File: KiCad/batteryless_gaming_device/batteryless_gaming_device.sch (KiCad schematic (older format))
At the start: 0 parts

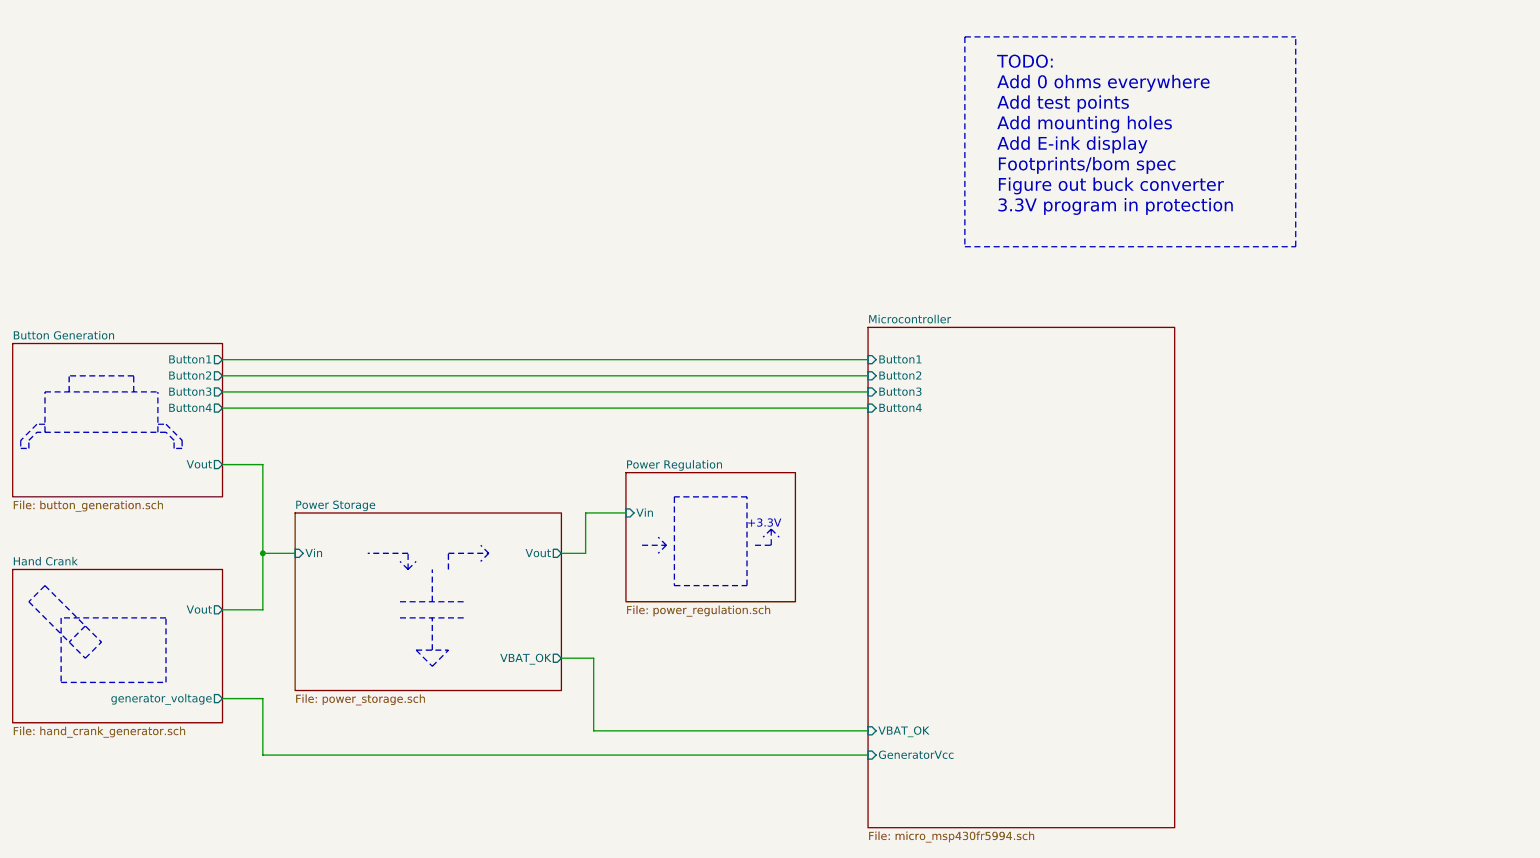
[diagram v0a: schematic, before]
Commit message: k
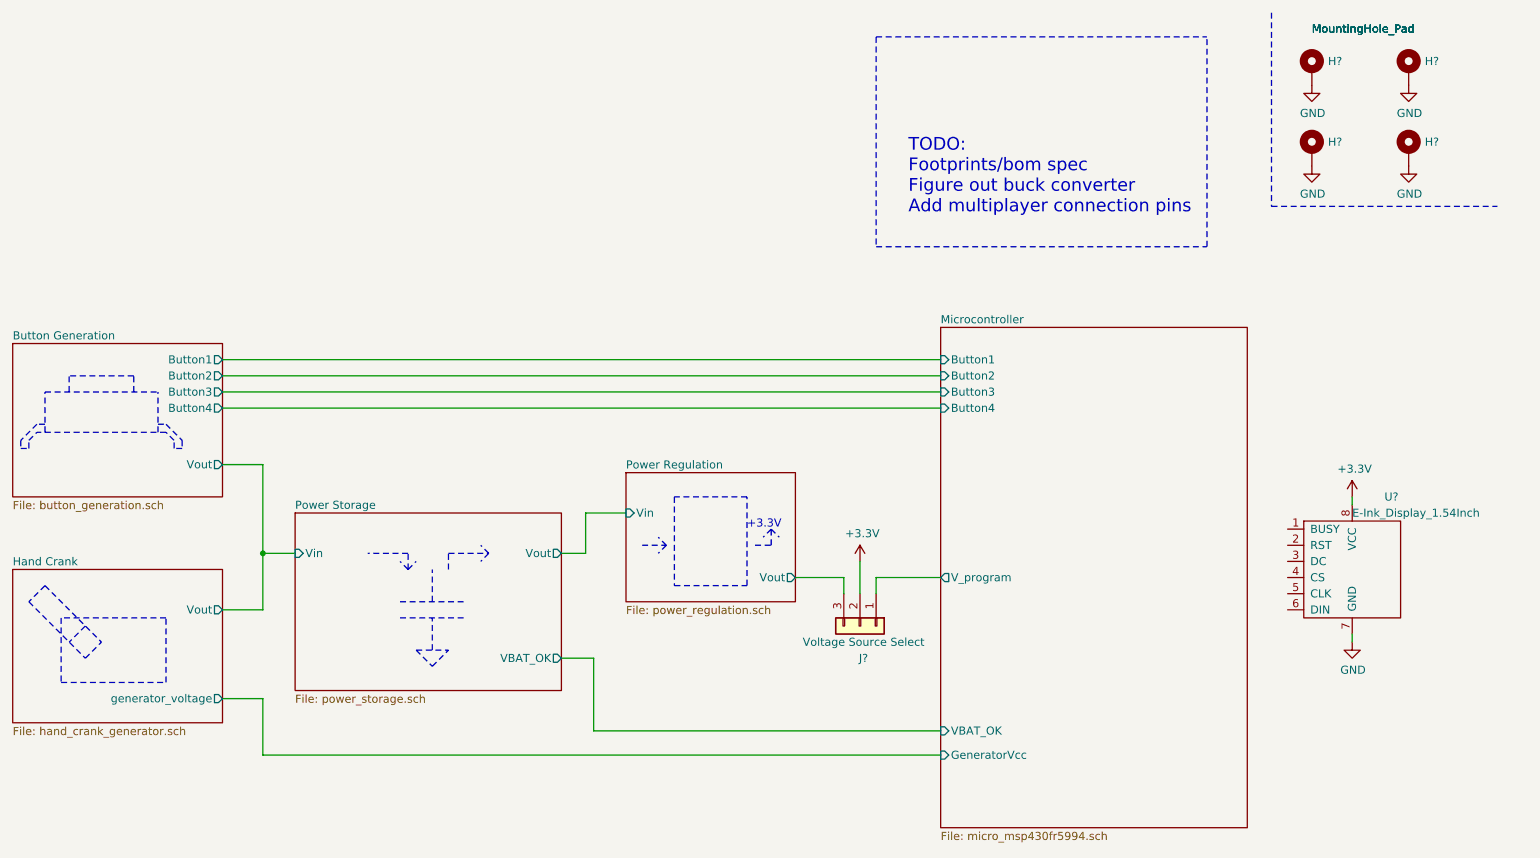
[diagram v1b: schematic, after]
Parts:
- added H? (x4): MountingHole_Pad, symbol Mechanical:MountingHole_Pad
- added J?: Voltage Source Select, symbol Connector_Generic:Conn_01x03
- added U?: E-Ink_Display_1.54Inch, symbol batteryless_gaming_device-rescue:E-Ink_Display_1.54Inch
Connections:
- new net +3V3: J?.2 (Pin_2), U?.8 (VCC)
- new net GND: H?.1, H?.1, H?.1, H?.1, U?.7 (GND)
- new net Microcontroller/V_program: J?.1 (Pin_1)
- new net Power Regulation/Vout: J?.3 (Pin_3)
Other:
- note added: "TODO:\nFootprints/bom spec\nFigure out buck converter\nAdd multiplayer connection pins"
- note removed: "TODO:\nAdd 0 ohms everywhere\nAdd test points\nAdd mounting holes\nAdd E-ink display\nFootprints/bom spec\nFigure out buck converter\n3.3V program in protection"
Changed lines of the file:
@@
 $EndSheet
 $Sheet
-S 6600 2450 1900 3100
+S 7050 2450 1900 3100
 U 61926AE2
 F0 "Microcontroller" 50
 F1 "micro_msp430fr5994.sch" 50
-F2 "Button1" I L 6600 2650 50
-F3 "Button2" I L 6600 2750 50
-F4 "Button3" I L 6600 2850 50
-F5 "Button4" I L 6600 2950 50
-F6 "GeneratorVcc" I L 6600 5100 50
-F7 "VBAT_OK" I L 6600 4950 50
+F2 "Button1" I L 7050 2650 50
+F3 "Button2" I L 7050 2750 50
+F4 "Button3" I L 7050 2850 50
+F5 "Button4" I L 7050 2950 50
+F6 "GeneratorVcc" I L 7050 5100 50
+F7 "VBAT_OK" I L 7050 4950 50
+F8 "V_program" O L 7050 4000 50
 $EndSheet
 Wire Wire Line
@@
 F1 "power_regulation.sch" 50
 F2 "Vin" I L 5100 3600 50
+F3 "Vout" O R 6150 4000 50
 $EndSheet
 Wire Wire Line
@@
 	5200 3800 5350 3800
 Wire Wire Line
-	2600 2950 6600 2950
-Wire Wire Line
-	2600 2850 6600 2850
-Wire Wire Line
-	2600 2750 6600 2750
-Wire Wire Line
-	2600 2650 6600 2650
+	2600 2950 7050 2950
+Wire Wire Line
+	2600 2850 7050 2850
+Wire Wire Line
+	2600 2750 7050 2750
+Wire Wire Line
+	2600 2650 7050 2650
 Wire Wire Line
 	2600 4750 2850 4750
@@
 	2850 4750 2850 5100
 Wire Wire Line
-	2850 5100 6600 5100
+	2850 5100 7050 5100
 Wire Wire Line
 	4700 4500 4900 4500
@@
 	4900 4500 4900 4950
 Wire Wire Line
-	4900 4950 6600 4950
-Text Notes 7400 1750 0    79   ~ 0
-TODO:\nAdd 0 ohms everywhere\nAdd test points\nAdd mounting holes\nAdd E-ink display\nFootprints/bom spec\nFigure out buck converter\n3.3V program in protection
-Wire Notes Line
-	7200 650  7200 1950
-Wire Notes Line
-	7200 1950 9250 1950
-Wire Notes Line
-	9250 1950 9250 650
-Wire Notes Line
-	7200 650  9250 650
+	4900 4950 7050 4950
+Text Notes 6850 1750 0    79   ~ 0
+TODO:\nFootprints/bom spec\nFigure out buck converter\nAdd multiplayer connection pins
+Wire Notes Line
+	6650 650  6650 1950
+Wire Notes Line
+	6650 1950 8700 1950
+Wire Notes Line
+	8700 1950 8700 650
+Wire Notes Line
+	6650 650  8700 650
+$Comp
+L Connector_Generic:Conn_01x03 J?
+U 1 1 61979531
+P 6550 4300
+F 0 "J?" V 6750 4350 50  0000 R CNN
+F 1 "Voltage Source Select" V 6650 4700 50  0000 R CNN
+F 2 "" H 6550 4300 50  0001 C CNN
+F 3 "~" H 6550 4300 50  0001 C CNN
+	1    6550 4300
+	0    1    1    0
+$EndComp
+Wire Wire Line
+	6150 4000 6450 4000
+Wire Wire Line
+	6450 4000 6450 4100
+Wire Wire Line
+	7050 4000 6650 4000
+Wire Wire Line
+	6650 4000 6650 4100
+Wire Wire Line
+	6550 4100 6550 3900
+$Comp
+L power:+3.3V #PWR?
+U 1 1 61980457
+P 6550 3900
+AR Path="/61926AE2/61980457" Ref="#PWR?"  Part="1"
+AR Path="/61980457" Ref="#PWR?"  Part="1"
+F 0 "#PWR?" H 6550 3750 50  0001 C CNN
+F 1 "+3.3V" H 6565 4073 50  0000 C CNN
+F 2 "" H 6550 3900 50  0001 C CNN
+F 3 "" H 6550 3900 50  0001 C CNN
+	1    6550 3900
+	1    0    0    -1
+$EndComp
+$Comp
+L batteryless_gaming_device-rescue:E-Ink_Display_1.54Inch U?
+U 1 1 61986176
+P 9550 3650
+F 0 "U?" H 9800 3800 50  0000 L CNN
+F 1 "E-Ink_Display_1.54Inch" H 9600 3700 50  0000 L CNN
+F 2 "" H 9550 4150 50  0001 C CNN
+F 3 "" H 9550 4150 50  0001 C CNN
+	1    9550 3650
+	1    0    0    -1
+$EndComp
+$Comp
+L power:GND #PWR?
+U 1 1 61988A0E
+P 9600 4400
+AR Path="/61926AE2/61988A0E" Ref="#PWR?"  Part="1"
+AR Path="/61988A0E" Ref="#PWR?"  Part="1"
+F 0 "#PWR?" H 9600 4150 50  0001 C CNN
+F 1 "GND" H 9605 4227 50  0000 C CNN
+F 2 "" H 9600 4400 50  0001 C CNN
+F 3 "" H 9600 4400 50  0001 C CNN
+	1    9600 4400
+	1    0    0    -1
+$EndComp
+Wire Wire Line
+	9600 4400 9600 4350
+$Comp
+L power:+3.3V #PWR?
+U 1 1 6198A1ED
+P 9600 3500
+AR Path="/61926AE2/6198A1ED" Ref="#PWR?"  Part="1"
+AR Path="/6198A1ED" Ref="#PWR?"  Part="1"
+F 0 "#PWR?" H 9600 3350 50  0001 C CNN
+F 1 "+3.3V" H 9615 3673 50  0000 C CNN
+F 2 "" H 9600 3500 50  0001 C CNN
+F 3 "" H 9600 3500 50  0001 C CNN
+	1    9600 3500
+	1    0    0    -1
+$EndComp
+Wire Wire Line
+	9600 3500 9600 3550
+$Comp
+L Mechanical:MountingHole_Pad H?
+U 1 1 6198BDFD
+P 9350 850
+F 0 "H?" H 9450 899 50  0000 L CNN
+F 1 "MountingHole_Pad" H 9350 1100 50  0000 L CNN
+F 2 "" H 9350 850 50  0001 C CNN
+F 3 "~" H 9350 850 50  0001 C CNN
+	1    9350 850
+	1    0    0    -1
+$EndComp
+$Comp
+L Mechanical:MountingHole_Pad H?
+U 1 1 6198CE4F
+P 9950 850
+F 0 "H?" H 10050 899 50  0000 L CNN
+F 1 "MountingHole_Pad" H 9350 1100 50  0000 L CNN
+F 2 "" H 9950 850 50  0001 C CNN
+F 3 "~" H 9950 850 50  0001 C CNN
+	1    9950 850
+	1    0    0    -1
+$EndComp
+$Comp
+L Mechanical:MountingHole_Pad H?
+U 1 1 6198D15F
+P 9350 1350
+F 0 "H?" H 9450 1399 50  0000 L CNN
+F 1 "MountingHole_Pad" H 9350 2100 50  0000 L CNN
+F 2 "" H 9350 1350 50  0001 C CNN
+F 3 "~" H 9350 1350 50  0001 C CNN
+	1    9350 1350
+	1    0    0    -1
+$EndComp
+$Comp
+L Mechanical:MountingHole_Pad H?
+U 1 1 6198D37A
+P 9950 1350
+F 0 "H?" H 10050 1399 50  0000 L CNN
+F 1 "MountingHole_Pad" H 9350 2100 50  0000 L CNN
+F 2 "" H 9950 1350 50  0001 C CNN
+F 3 "~" H 9950 1350 50  0001 C CNN
+	1    9950 1350
+	1    0    0    -1
+$EndComp
+$Comp
+L power:GND #PWR?
+U 1 1 6198DDE0
+P 9350 1450
+AR Path="/61926AE2/6198DDE0" Ref="#PWR?"  Part="1"
+AR Path="/6198DDE0" Ref="#PWR?"  Part="1"
+F 0 "#PWR?" H 9350 1200 50  0001 C CNN
+F 1 "GND" H 9355 1277 50  0000 C CNN
+F 2 "" H 9350 1450 50  0001 C CNN
+F 3 "" H 9350 1450 50  0001 C CNN
+	1    9350 1450
+	1    0    0    -1
+$EndComp
+$Comp
+L power:GND #PWR?
+U 1 1 6198E313
+P 9950 1450
+AR Path="/61926AE2/6198E313" Ref="#PWR?"  Part="1"
+AR Path="/6198E313" Ref="#PWR?"  Part="1"
+F 0 "#PWR?" H 9950 1200 50  0001 C CNN
+F 1 "GND" H 9955 1277 50  0000 C CNN
+F 2 "" H 9950 1450 50  0001 C CNN
+F 3 "" H 9950 1450 50  0001 C CNN
+	1    9950 1450
+	1    0    0    -1
+$EndComp
+$Comp
+L power:GND #PWR?
+U 1 1 6198E5F3
+P 9350 950
+AR Path="/61926AE2/6198E5F3" Ref="#PWR?"  Part="1"
+AR Path="/6198E5F3" Ref="#PWR?"  Part="1"
+F 0 "#PWR?" H 9350 700 50  0001 C CNN
+F 1 "GND" H 9355 777 50  0000 C CNN
+F 2 "" H 9350 950 50  0001 C CNN
+F 3 "" H 9350 950 50  0001 C CNN
+	1    9350 950
+	1    0    0    -1
+$EndComp
+$Comp
+L power:GND #PWR?
+U 1 1 6198E95A
+P 9950 950
+AR Path="/61926AE2/6198E95A" Ref="#PWR?"  Part="1"
+AR Path="/6198E95A" Ref="#PWR?"  Part="1"
+F 0 "#PWR?" H 9950 700 50  0001 C CNN
+F 1 "GND" H 9955 777 50  0000 C CNN
+F 2 "" H 9950 950 50  0001 C CNN
+F 3 "" H 9950 950 50  0001 C CNN
+	1    9950 950
+	1    0    0    -1
+$EndComp
+Wire Notes Line
+	9100 500  9100 1700
+Wire Notes Line
+	9100 1700 10500 1700
 $EndSCHEMATC
